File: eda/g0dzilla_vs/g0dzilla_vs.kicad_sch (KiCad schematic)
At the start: 50 parts, among them J1 Battery_Conn, J2 01x02, J3 01x02, J4 01x02, J5 01x02, SW1 SW_SPDT_SS12D00G, U1 ESP32-WEMOS-LOLIN32-LITE

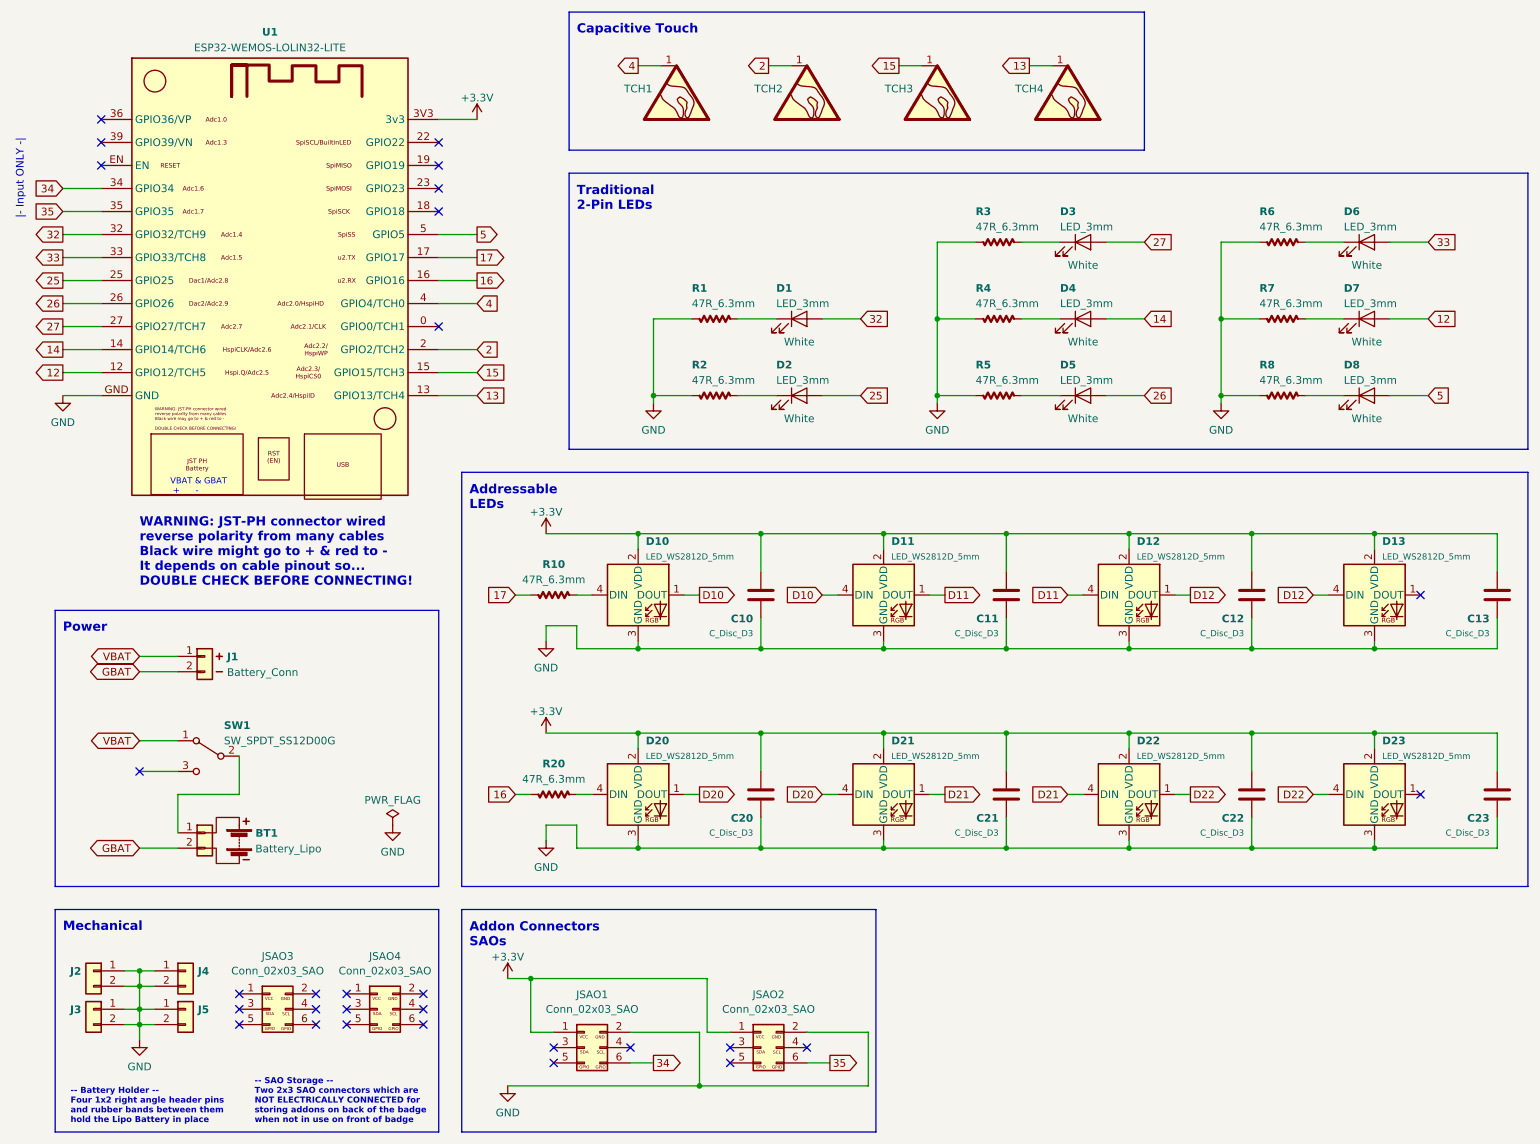
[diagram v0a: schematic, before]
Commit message: pcb updates
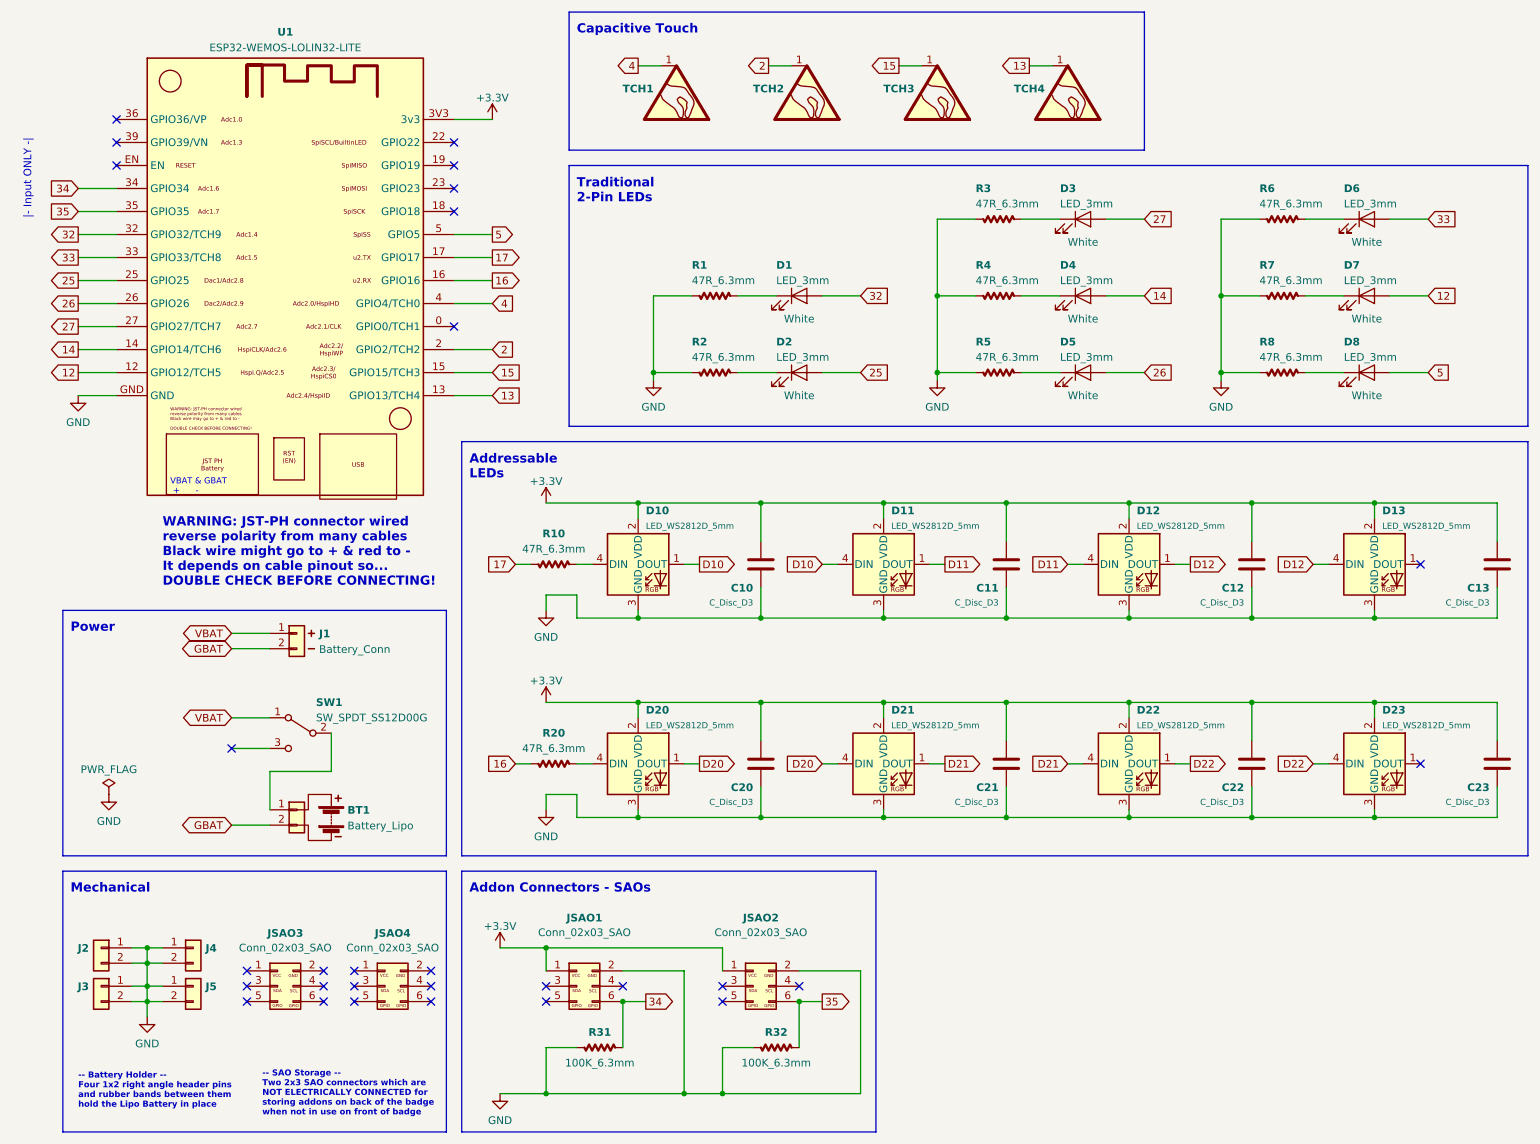
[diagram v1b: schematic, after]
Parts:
- added R31, R32: 100K_6.3mm, 0_local:R_Axial_DIN0207_L6.3_D2.5_P7.62_Horiz_back, symbol 0_local:R_Axial_Z_L6.3
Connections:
- net 34: now also R31.1
- net 35: now also R32.1
- net GND: now also R31.2, R32.2
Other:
- note added: "Addon Connectors - SAOs"
- note removed: "Addon Connectors SAOs"
- moved on the sheet: BT1, C10, C11, C12, C13, C20, C21, C22, C23, D1, D10, D11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
